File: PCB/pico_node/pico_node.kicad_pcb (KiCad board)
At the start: 2 copper layers, 107.3 x 53.3 mm, 19 parts, among them J1 INMP441, J2 NEO-6M, J3 MD-CD42, J4 RESET_POWER_SW, J5 UART0_DEBUG, J6 UART1_DEBUG, J7 BATTERY, J8 BUCK_5V, Q1 BC547, U1 NRF24L01_Breakout, U2 AMS1117-3.3

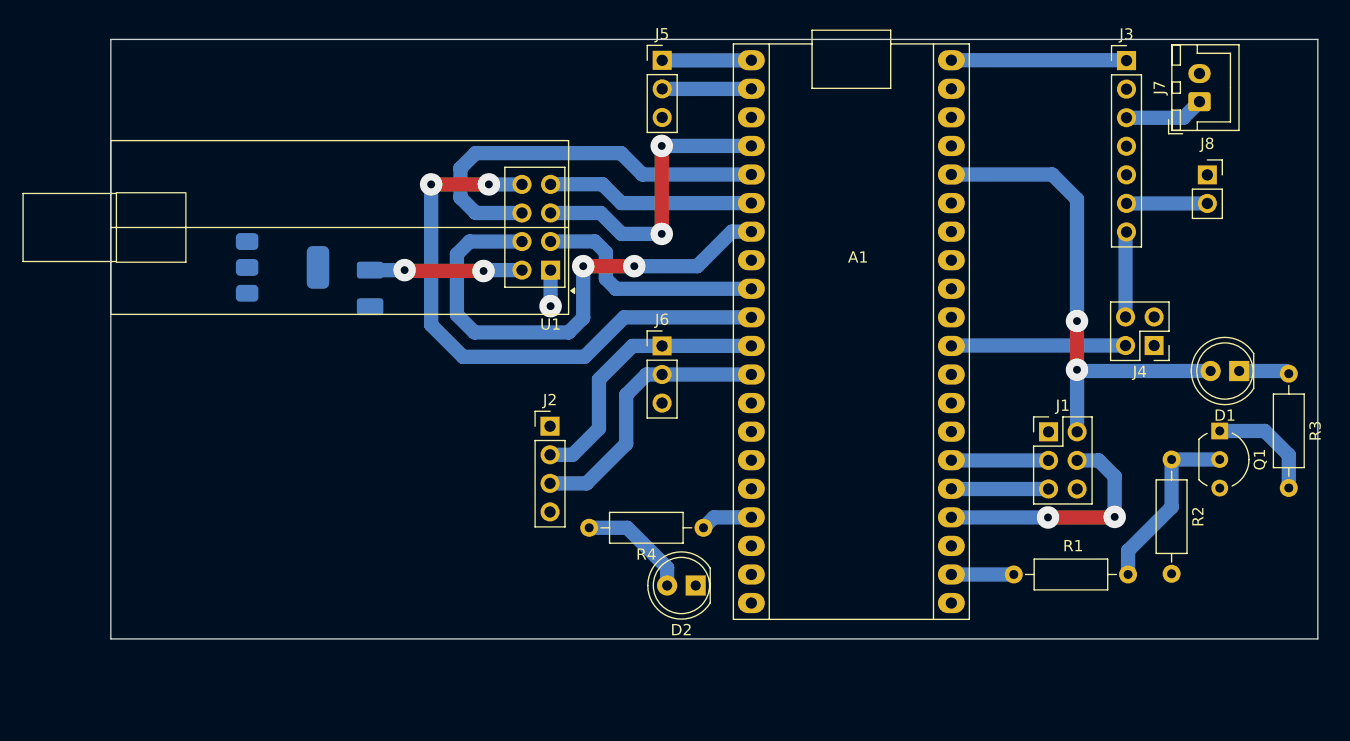
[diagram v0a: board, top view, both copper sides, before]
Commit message: Update on pico_node pcb
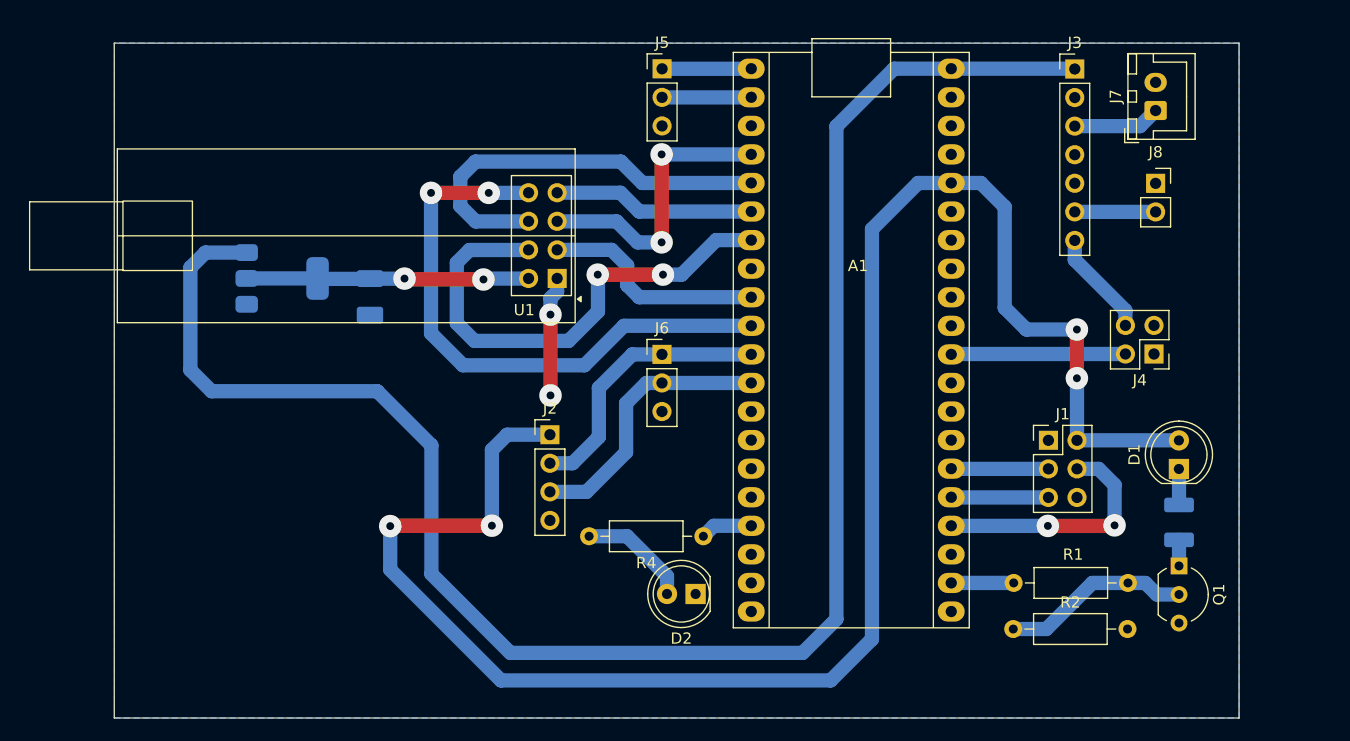
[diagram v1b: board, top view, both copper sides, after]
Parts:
- R3: footprint Resistor_THT:R_Axial_DIN0207_L6.3mm_D2.5mm_P10.16mm_Horizontal -> Resistor_SMD:R_1210_3225Metric_Pad1.30x2.65mm_HandSolder; moved to B.Cu
- moved R2 20.6 mm to (175.9, 90.1), turned to 0 degrees
- moved R3 16.4 mm to (190.7, 80.6)
- moved Q1 12.5 mm to (190.7, 84.5)
- moved D1 10.2 mm to (190.7, 75.9), turned to 90 degrees
- moved J3 4.66 mm to (181.4, 40.3)
- moved J8 4.66 mm to (188.6, 50.5)
- moved J7 3.98 mm to (188.6, 44.0)
- moved U2 0.98 mm to (110.9, 58.9)
- moved U1 0.94 mm to (136.9, 55.1)
- moved R1 0.75 mm to (176.0, 86.0)
- moved J2 0.75 mm to (134.7, 72.8)
- moved J5 0.75 mm to (144.7, 40.3)
- moved A1 0.75 mm to (152.6, 40.3)
- moved C1 0.75 mm to (118.7, 60.6)
- moved D2 0.75 mm to (147.7, 87.0)
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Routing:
- net VBUS: track 15.6 -> 157.6 mm
- net +3.3V: track 44.7 -> 159.9 mm, vias 2 -> 4
- net Net-(C1-+): track 13.0 -> 24.6 mm
- net Net-(Q1-C): track 9.96 -> 2.32 mm
- net GND: track 3.20 -> 10.6 mm, vias 1 -> 2
- net /POWER_KEY: track 7.59 -> 9.42 mm
- net Net-(R3-+): track 4.51 -> 3.20 mm
- net /GP6: track 20.9 -> 20.0 mm
- net Net-(Q1-B): track 16.1 -> 16.9 mm
- net Net-(J3-Pin_3): track 7.08 -> 7.77 mm
- net /GP7: track 51.7 -> 52.3 mm
- net /GP3: track 35.9 -> 36.5 mm
- net /GP2: track 26.4 -> 25.9 mm
- net /GP4: track 18.5 -> 18.0 mm
- added copper zone on B.Cu, net GND
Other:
- board size 107.3 x 53.3 mm -> 100 x 60 mm
